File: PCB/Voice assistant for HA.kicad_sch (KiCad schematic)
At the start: 31 parts, among them J1 Conn_01x06_Pin, J2 Screw_Terminal_01x02, J3 Conn_01x03_Pin, J4 Conn_01x03_Pin, J5 Conn_01x03_Pin, J6 Conn_01x03_Pin, U1 AMS1117-3.3, U2 ESP32-S3-WROOM-1, U3 MAX98357A

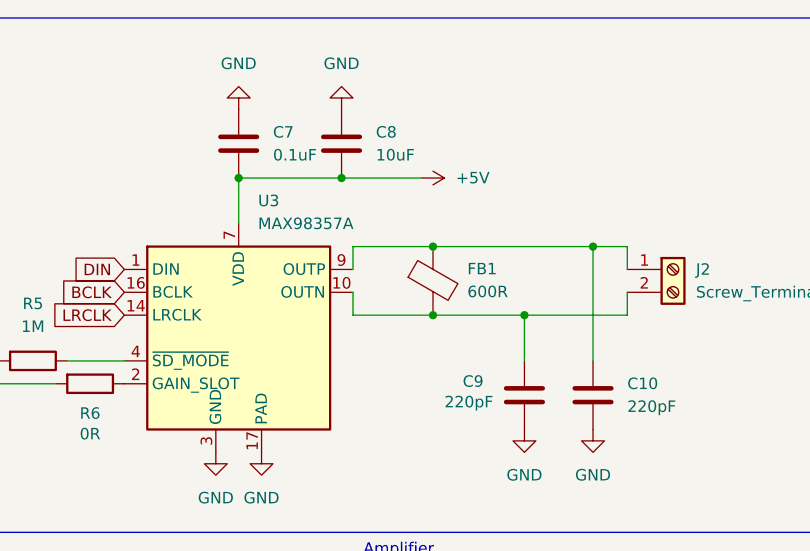
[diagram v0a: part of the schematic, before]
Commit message: post-assembly adjustments
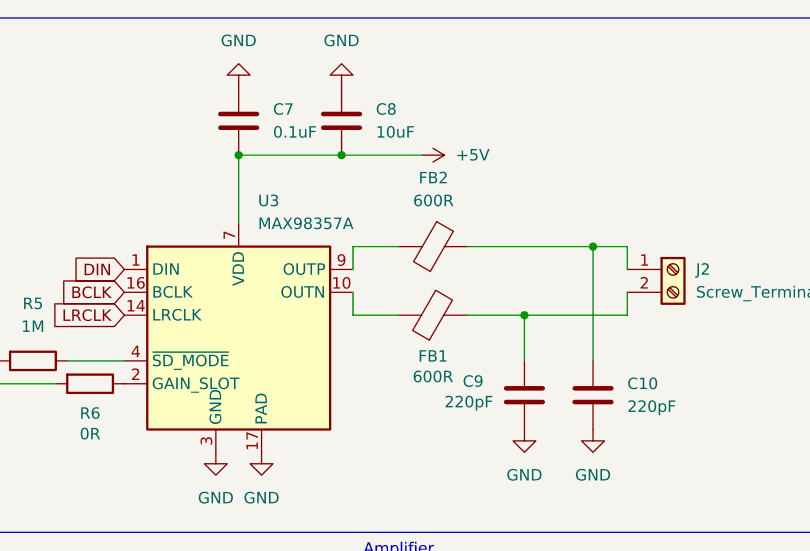
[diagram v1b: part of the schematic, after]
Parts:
- added FB2: 600R, Inductor_SMD:L_0805_2012Metric, symbol Device:FerriteBead
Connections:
- net at C10.1, J2.1 (Pin_1): now also FB2.1; no longer FB1.1, U3.9 (OUTP)
- net at C9.1, FB1.2, J2.2 (Pin_2): no longer U3.10 (OUTN)
- new net: FB1.1, U3.10 (OUTN)
- new net: FB2.2, U3.9 (OUTP)
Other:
- moved on the sheet: C7, C8, FB1
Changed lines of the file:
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@@
 	)
 	(junction
-		(at 74.93 29.21)
-		(diameter 0)
-		(color 0 0 0 0)
-	)
-	(junction
-		(at 214.63 50.8)
-		(diameter 0)
-		(color 0 0 0 0)
-	)
-	(junction
-		(at 214.63 43.18)
+		(at 232.41 43.18)
 		(diameter 0)
 		(color 0 0 0 0)
 	)
 	(junction
-		(at 232.41 43.18)
+		(at 74.93 29.21)
 		(diameter 0)
 		(color 0 0 0 0)
 	)
 	(junction
-		(at 193.04 35.56)
+		(at 193.04 33.02)
 		(diameter 0)
 		(color 0 0 0 0)
 	)
 	(junction
-		(at 204.47 35.56)
+		(at 204.47 33.02)
 		(diameter 0)
 		(color 0 0 0 0)
@@
 	)
 	(junction
-		(at 45.72 138.43)
+		(at 224.79 50.8)
 		(diameter 0)
 		(color 0 0 0 0)
 	)
 	(junction
-		(at 224.79 50.8)
+		(at 45.72 138.43)
 		(diameter 0)
 		(color 0 0 0 0)
@@
 	(wire
 		(pts
-			(xy 166.37 58.42) (xy 172.72 58.42)
+			(xy 218.44 50.8) (xy 224.79 50.8)
 		)
 		(stroke
@@
 	(wire
 		(pts
-			(xy 74.93 29.21) (xy 77.47 29.21)
+			(xy 166.37 58.42) (xy 172.72 58.42)
 		)
 		(stroke
@@
 	(wire
 		(pts
-			(xy 115.57 151.13) (xy 123.19 151.13)
+			(xy 205.74 43.18) (xy 210.82 43.18)
 		)
 		(stroke
@@
 	(wire
 		(pts
-			(xy 45.72 147.32) (xy 41.91 147.32)
+			(xy 74.93 29.21) (xy 77.47 29.21)
 		)
 		(stroke
@@
 	(wire
 		(pts
-			(xy 173.99 55.88) (xy 180.34 55.88)
+			(xy 115.57 151.13) (xy 123.19 151.13)
 		)
 		(stroke
@@
 	(wire
 		(pts
-			(xy 54.61 29.21) (xy 57.15 29.21)
+			(xy 45.72 147.32) (xy 41.91 147.32)
 		)
 		(stroke
@@
 	(wire
 		(pts
-			(xy 214.63 50.8) (xy 224.79 50.8)
+			(xy 173.99 55.88) (xy 180.34 55.88)
 		)
 		(stroke
@@
 	(wire
 		(pts
-			(xy 205.74 50.8) (xy 214.63 50.8)
+			(xy 54.61 29.21) (xy 57.15 29.21)
 		)
 		(stroke
@@
 	(wire
 		(pts
-			(xy 204.47 35.56) (xy 213.36 35.56)
+			(xy 218.44 43.18) (xy 232.41 43.18)
+		)
+		(stroke
+			(width 0)
+			(type default)
+		)
+	)
+	(wire
+		(pts
+			(xy 204.47 33.02) (xy 213.36 33.02)
 		)
 		(stroke
@@
 	(wire
 		(pts
-			(xy 193.04 35.56) (xy 193.04 40.64)
+			(xy 193.04 33.02) (xy 193.04 40.64)
 		)
 		(stroke
@@
 	(wire
 		(pts
-			(xy 205.74 43.18) (xy 214.63 43.18)
+			(xy 205.74 50.8) (xy 210.82 50.8)
 		)
 		(stroke
@@
 	(wire
 		(pts
-			(xy 193.04 35.56) (xy 204.47 35.56)
-		)
-		(stroke
-			(width 0)
-			(type default)
-		)
-	)
-	(wire
-		(pts
-			(xy 214.63 43.18) (xy 232.41 43.18)
+			(xy 193.04 33.02) (xy 204.47 33.02)
 		)
 		(stroke
@@
 	(symbol
 		(lib_id "Device:FerriteBead")
-		(at 214.63 46.99 0)
+		(at 214.63 50.8 90)
 		(unit 1)
 		(exclude_from_sim no)
@@
 		(on_board yes)
 		(dnp no)
-		(fields_autoplaced yes)
 		(property "Reference" "FB1"
-			(at 218.44 45.6691 0)
+			(at 214.63 55.372 90)
 			(effects
 				(font
 					(size 1.27 1.27)
 				)
-				(justify left)
 			)
 		)
 		(property "Value" "600R"
-			(at 218.44 48.2091 0)
+			(at 214.63 57.658 90)
 			(effects
 				(font
 					(size 1.27 1.27)
 				)
-				(justify left)
 			)
 		)
 		(property "Footprint" "Inductor_SMD:L_0805_2012Metric"
-			(at 212.852 46.99 90)
+			(at 214.63 52.578 90)
 			(effects
 				(font
@@
 		)
 		(property "Datasheet" "~"
-			(at 214.63 46.99 0)
+			(at 214.63 50.8 0)
 			(effects
 				(font
@@
 		)
 		(property "Description" "Ferrite bead"
-			(at 214.63 46.99 0)
+			(at 214.63 50.8 0)
 			(effects
 				(font
@@
 	(symbol
 		(lib_id "power:+5V")
-		(at 213.36 35.56 270)
+		(at 213.36 33.02 270)
 		(unit 1)
 		(exclude_from_sim no)
@@
 		(fields_autoplaced yes)
 		(property "Reference" "#PWR023"
-			(at 209.55 35.56 0)
+			(at 209.55 33.02 0)
 			(effects
 				(font
@@
 		)
 		(property "Value" "+5V"
-			(at 217.17 35.5599 90)
+			(at 217.17 33.0199 90)
 			(effects
 				(font
@@
 		)
 		(property "Footprint" ""
-			(at 213.36 35.56 0)
+			(at 213.36 33.02 0)
 			(effects
 				(font
@@
 		)
 		(property "Datasheet" ""
-			(at 213.36 35.56 0)
+			(at 213.36 33.02 0)
 			(effects
 				(font
@@
 		)
 		(property "Description" "Power symbol creates a global label with name \"+5V\""
-			(at 213.36 35.56 0)
+			(at 213.36 33.02 0)
 			(effects
 				(font
@@
 	(symbol
 		(lib_id "Device:C")
-		(at 204.47 31.75 0)
+		(at 204.47 29.21 0)
 		(unit 1)
 		(exclude_from_sim no)
@@
 		(fields_autoplaced yes)
 		(property "Reference" "C8"
-			(at 208.28 30.4799 0)
+			(at 208.28 27.9399 0)
 			(effects
 				(font
@@
 		)
 		(property "Value" "10uF"
-			(at 208.28 33.0199 0)
+			(at 208.28 30.4799 0)
 			(effects
 				(font
@@
 		)
 		(property "Footprint" "Capacitor_SMD:C_0805_2012Metric"
-			(at 205.4352 35.56 0)
+			(at 205.4352 33.02 0)
 			(effects
 				(font
@@
 		)
 		(property "Datasheet" "~"
-			(at 204.47 31.75 0)
+			(at 204.47 29.21 0)
 			(effects
 				(font
@@
 		)
 		(property "Description" "Unpolarized capacitor"
-			(at 204.47 31.75 0)
+			(at 204.47 29.21 0)
 			(effects
 				(font
@@
 	(symbol
 		(lib_id "Device:C")
-		(at 193.04 31.75 0)
+		(at 193.04 29.21 0)
 		(unit 1)
 		(exclude_from_sim no)
@@
 		(fields_autoplaced yes)
 		(property "Reference" "C7"
-			(at 196.85 30.4799 0)
+			(at 196.85 27.9399 0)
 			(effects
 				(font
@@
 		)
 		(property "Value" "0.1uF"
-			(at 196.85 33.0199 0)
+			(at 196.85 30.4799 0)
 			(effects
 				(font
@@
 		)
 		(property "Footprint" "Capacitor_SMD:C_0805_2012Metric"
-			(at 194.0052 35.56 0)
+			(at 194.0052 33.02 0)
 			(effects
 				(font
@@
 		)
 		(property "Datasheet" "~"
-			(at 193.04 31.75 0)
+			(at 193.04 29.21 0)
 			(effects
 				(font
@@
 		)
 		(property "Description" "Unpolarized capacitor"
-			(at 193.04 31.75 0)
+			(at 193.04 29.21 0)
 			(effects
 				(font
@@
 	)
 	(symbol
+		(lib_id "Device:FerriteBead")
+		(at 214.63 43.18 270)
+		(unit 1)
+		(exclude_from_sim no)
+		(in_bom yes)
+		(on_board yes)
+		(dnp no)
+		(fields_autoplaced yes)
+		(property "Reference" "FB2"
+			(at 214.6808 35.56 90)
+			(effects
+				(font
+					(size 1.27 1.27)
+				)
+			)
+		)
+		(property "Value" "600R"
+			(at 214.6808 38.1 90)
+			(effects
+				(font
+					(size 1.27 1.27)
+				)
+			)
+		)
+		(property "Footprint" "Inductor_SMD:L_0805_2012Metric"
+			(at 214.63 41.402 90)
+			(effects
+				(font
+					(size 1.27 1.27)
+				)
+				(hide yes)
+			)
+		)
+		(property "Datasheet" "~"
+			(at 214.63 43.18 0)
+			(effects
+				(font
+					(size 1.27 1.27)
+				)
+				(hide yes)
+			)
+		)
+		(property "Description" "Ferrite bead"
+			(at 214.63 43.18 0)
+			(effects
+				(font
+					(size 1.27 1.27)
+				)
+				(hide yes)
+			)
+		)
+		(pin "1"
+		)
+		(pin "2"
+		)
+		(instances
+			(project "Voice assistant for HA"
+				(path "/adef892d-59f2-4a90-8cdb-a41d078b638c"
+					(reference "FB2")
+					(unit 1)
+				)
+			)
+		)
+	)
+	(symbol
 		(lib_id "TS-1088-AR02016:TS-1088-AR02016")
 		(at 38.1 138.43 0)
@@
 	(symbol
 		(lib_id "power:GND")
-		(at 193.04 27.94 180)
+		(at 193.04 25.4 180)
 		(unit 1)
 		(exclude_from_sim no)
@@
 		(fields_autoplaced yes)
 		(property "Reference" "#PWR024"
-			(at 193.04 21.59 0)
+			(at 193.04 19.05 0)
 			(effects
 				(font
@@
 		)
 		(property "Value" "GND"
-			(at 193.04 22.86 0)
+			(at 193.04 20.32 0)
 			(effects
 				(font
@@
 		)
 		(property "Footprint" ""
-			(at 193.04 27.94 0)
+			(at 193.04 25.4 0)
 			(effects
 				(font
@@
 		)
 		(property "Datasheet" ""
-			(at 193.04 27.94 0)
+			(at 193.04 25.4 0)
 			(effects
 				(font
@@
 		)
 		(property "Description" "Power symbol creates a global label with name \"GND\" , ground"
-			(at 193.04 27.94 0)
+			(at 193.04 25.4 0)
 			(effects
 				(font
@@
 	(symbol
 		(lib_id "power:GND")
-		(at 204.47 27.94 180)
+		(at 204.47 25.4 180)
 		(unit 1)
 		(exclude_from_sim no)
@@
 		(fields_autoplaced yes)
 		(property "Reference" "#PWR025"
-			(at 204.47 21.59 0)
+			(at 204.47 19.05 0)
 			(effects
 				(font
@@
 		)
 		(property "Value" "GND"
-			(at 204.47 22.86 0)
+			(at 204.47 20.32 0)
 			(effects
 				(font
@@
 		)
 		(property "Footprint" ""
-			(at 204.47 27.94 0)
+			(at 204.47 25.4 0)
 			(effects
 				(font
@@
 		)
 		(property "Datasheet" ""
-			(at 204.47 27.94 0)
+			(at 204.47 25.4 0)
 			(effects
 				(font
@@
 		)
 		(property "Description" "Power symbol creates a global label with name \"GND\" , ground"
-			(at 204.47 27.94 0)
+			(at 204.47 25.4 0)
 			(effects
 				(font
